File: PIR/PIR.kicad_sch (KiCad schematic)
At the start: 32 parts, among them J1 FLASH, J2 PIR, J3 BUS, J4 Conn_01x04_Socket, Q1 BC846, Q2 BC846, Q3 BC857, SW1 tamper switch, U1 AP63203WU, U2 WT8266-S1

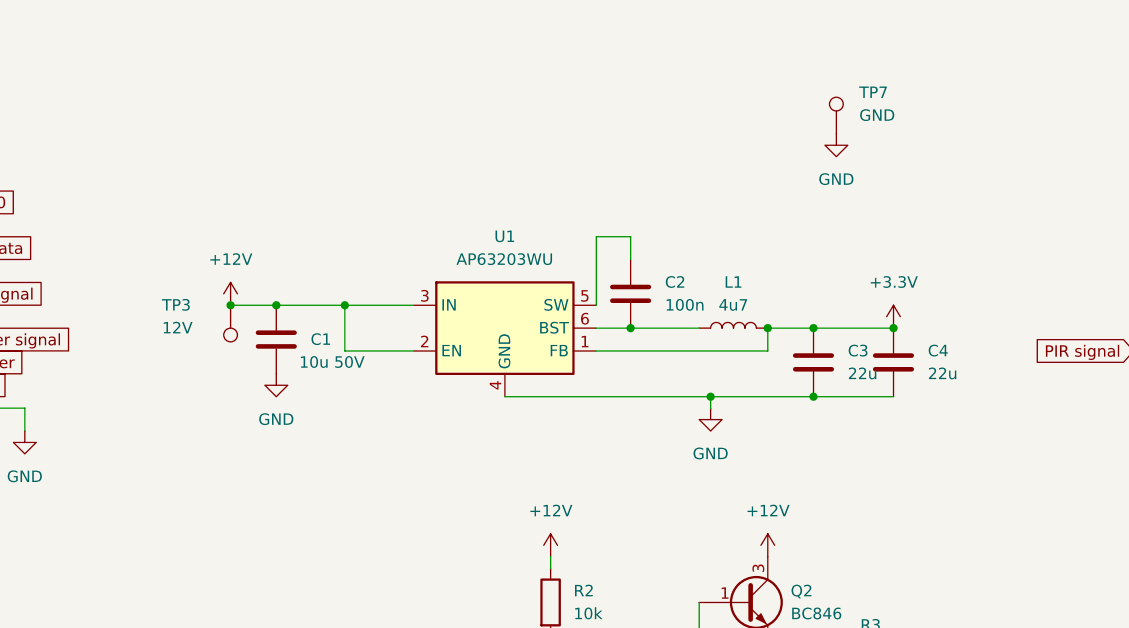
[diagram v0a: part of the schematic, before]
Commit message: Fix incident
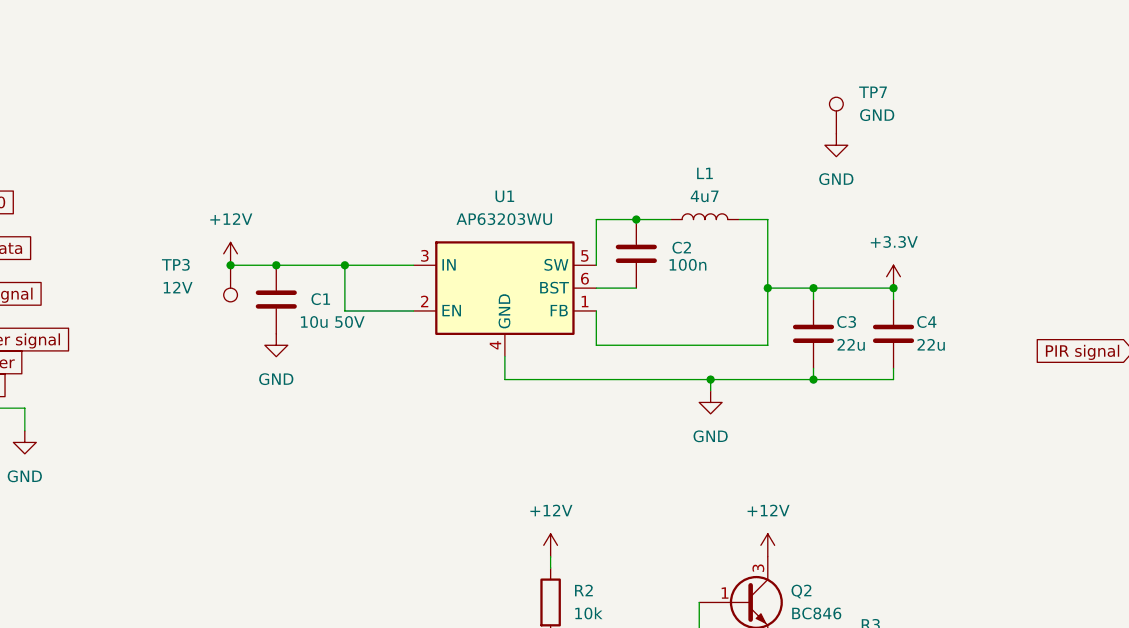
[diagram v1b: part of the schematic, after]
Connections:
- net at C2.2, L1.1: now also U1.5 (SW); no longer U1.6 (BST)
- net at C2.1: now also U1.6 (BST); no longer U1.5 (SW)
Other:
- moved on the sheet: C1, C2, C3, C4, L1, TP3, U1
